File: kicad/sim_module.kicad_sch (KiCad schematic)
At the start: 2 parts, among them J40 693043020611, U40 TPD3F303DPVR

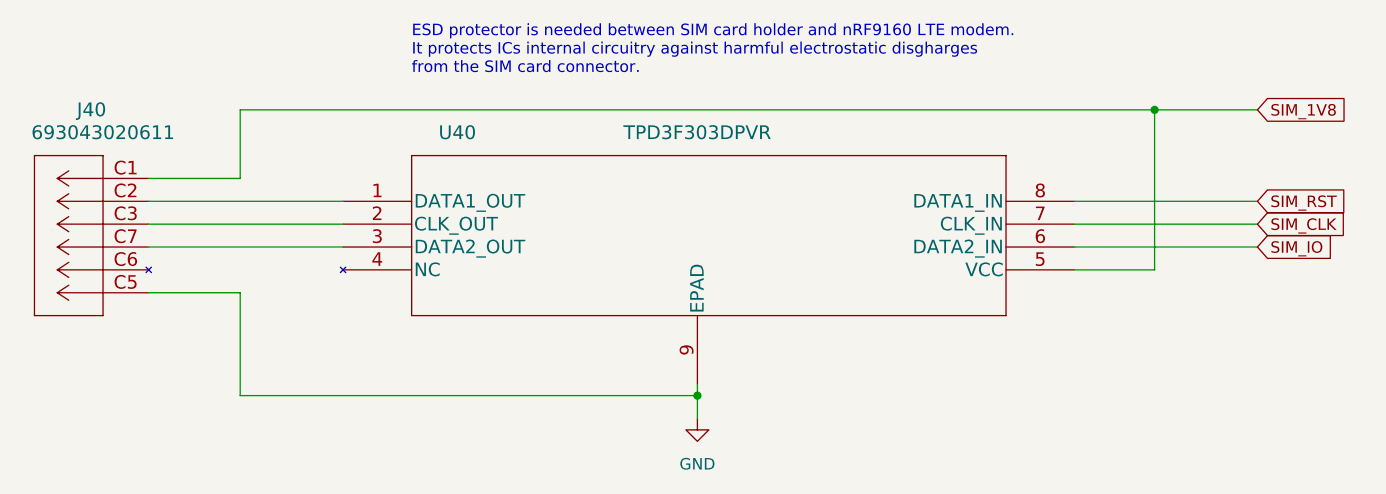
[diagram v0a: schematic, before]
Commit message: ESD change
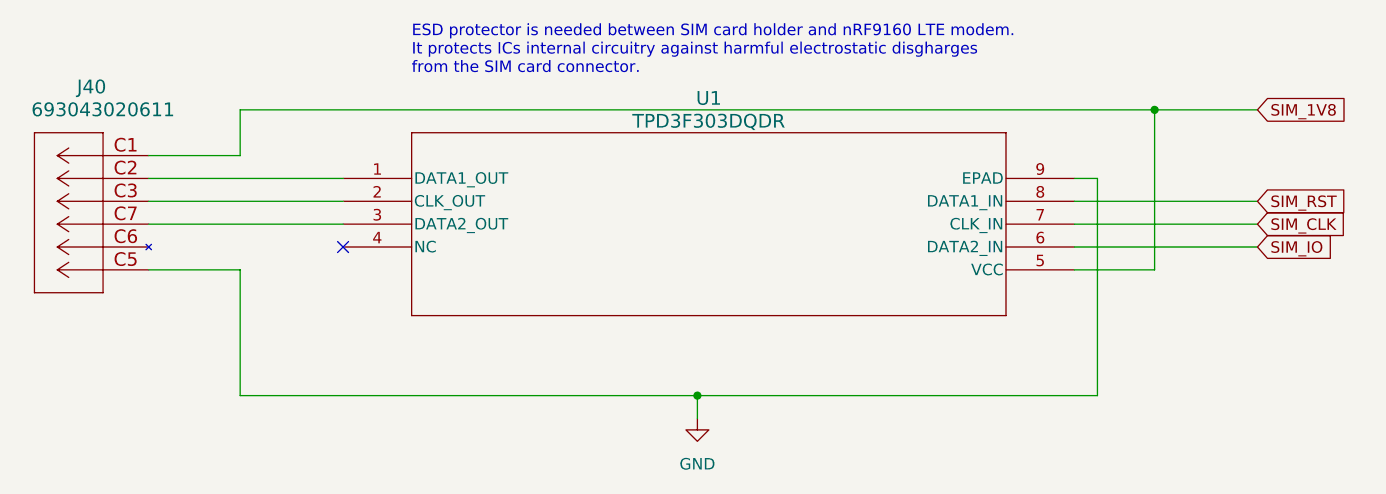
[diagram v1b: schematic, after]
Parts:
- removed U40: TPD3F303DPVR, TPD3F303DPVR:TPD3F303DPVR, symbol TPD3F303DPVR:TPD3F303DPVR
- added U1: TPD3F303DQDR, TPD3F303DQDR:TPD3F303DQDR, symbol TPD3F303DQDR:TPD3F303DQDR
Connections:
- net GND: now also U1.9 (EPAD)
- net SIM_1V8: now also U1.5 (VCC)
- net SIM_CLK: now also U1.7 (CLK_IN)
- net SIM_IO: now also U1.6 (DATA2_IN)
- net SIM_RST: now also U1.8 (DATA1_IN)
- net at J40.C2: now also U1.1 (DATA1_OUT)
- net at J40.C3: now also U1.2 (CLK_OUT)
- net at J40.C7: now also U1.3 (DATA2_OUT)
- no-connect marks 0 -> 1
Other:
- moved on the sheet: J40
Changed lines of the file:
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@@
   (junction (at 106.68 73.66) (diameter 0) (color 0 0 0 0)
   )
-  (wire (pts (xy 55.88 62.23) (xy 55.88 73.66))
+  (no_connect (at 67.31 57.15))
+  (wire (pts (xy 45.72 49.53) (xy 67.31 49.53))
+    (stroke (width 0) (type default))
+  )
+  (wire (pts (xy 55.88 59.69) (xy 55.88 73.66))
     (stroke (width 0) (type default))
   )
@@
     (stroke (width 0) (type default))
   )
-  (wire (pts (xy 45.72 49.53) (xy 55.88 49.53))
+  (wire (pts (xy 45.72 46.99) (xy 55.88 46.99))
+    (stroke (width 0) (type default))
+  )
+  (wire (pts (xy 148.59 49.53) (xy 151.13 49.53))
     (stroke (width 0) (type default))
   )
@@
     (stroke (width 0) (type default))
   )
+  (wire (pts (xy 45.72 52.07) (xy 67.31 52.07))
+    (stroke (width 0) (type default))
+  )
   (wire (pts (xy 55.88 41.91) (xy 157.48 41.91))
     (stroke (width 0) (type default))
   )
-  (wire (pts (xy 45.72 52.07) (xy 67.31 52.07))
+  (wire (pts (xy 151.13 73.66) (xy 106.68 73.66))
     (stroke (width 0) (type default))
   )
@@
     (stroke (width 0) (type default))
   )
-  (wire (pts (xy 55.88 49.53) (xy 55.88 41.91))
+  (wire (pts (xy 55.88 59.69) (xy 45.72 59.69))
     (stroke (width 0) (type default))
   )
-  (wire (pts (xy 45.72 57.15) (xy 67.31 57.15))
+  (wire (pts (xy 55.88 41.91) (xy 55.88 46.99))
     (stroke (width 0) (type default))
   )
-  (wire (pts (xy 106.68 72.39) (xy 106.68 73.66))
+  (wire (pts (xy 151.13 49.53) (xy 151.13 73.66))
     (stroke (width 0) (type default))
   )
   (wire (pts (xy 106.68 73.66) (xy 106.68 76.2))
-    (stroke (width 0) (type default))
-  )
-  (wire (pts (xy 45.72 62.23) (xy 55.88 62.23))
     (stroke (width 0) (type default))
   )
@@
     )
   )
-  (symbol (lib_id "693043020611:693043020611") (at 45.72 49.53 0) (mirror y) (unit 1)
+  (symbol (lib_id "693043020611:693043020611") (at 45.72 46.99 0) (mirror y) (unit 1)
     (in_bom yes) (on_board yes) (dnp no)
-    (property "Reference" "J40" (at 39.37 41.91 0)
+    (property "Reference" "J40" (at 39.37 39.37 0)
       (effects (font (size 1.524 1.524)))
     )
-    (property "Value" "693043020611" (at 40.64 44.45 0)
+    (property "Value" "693043020611" (at 40.64 41.91 0)
       (effects (font (size 1.524 1.524)))
     )
-    (property "Footprint" "693043020611:693043020611" (at 35.56 42.926 0)
+    (property "Footprint" "693043020611:693043020611" (at 35.56 40.386 0)
       (effects (font (size 1.524 1.524)) hide)
     )
-    (property "Datasheet" "" (at 45.72 49.53 0)
+    (property "Datasheet" "" (at 45.72 46.99 0)
       (effects (font (size 1.524 1.524)))
     )
-    (property "Digikey" "296-28299-1-ND" (at 45.72 49.53 0)
+    (property "Digikey" "296-28299-1-ND" (at 45.72 46.99 0)
       (effects (font (size 1.27 1.27)) hide)
     )
@@
         (path "/184b47ed-2c2b-4c02-be35-d18f4f4e5685/38627e9e-7096-4a1a-bc9e-0f2735fcbe8c"
           (reference "J40") (unit 1)
-        )
-      )
-    )
-  )
-  (symbol (lib_id "TPD3F303DPVR:TPD3F303DPVR") (at 67.31 52.07 0) (unit 1)
-    (in_bom yes) (on_board yes) (dnp no)
-    (property "Reference" "U40" (at 80.01 44.45 0)
-      (effects (font (size 1.524 1.524)))
-    )
-    (property "Value" "TPD3F303DPVR" (at 106.68 44.45 0)
-      (effects (font (size 1.524 1.524)))
-    )
-    (property "Footprint" "TPD3F303DPVR:TPD3F303DPVR" (at 26.67 58.166 0)
-      (effects (font (size 1.524 1.524)) hide)
-    )
-    (property "Datasheet" "" (at 67.31 52.07 0)
-      (effects (font (size 1.524 1.524)))
-    )
-    (property "Digikey" "732-5954-1-ND" (at 67.31 52.07 0)
-      (effects (font (size 1.27 1.27)) hide)
-    )
-    (pin "1")
-    (pin "2")
-    (pin "3")
-    (pin "4")
-    (pin "5")
-    (pin "6")
-    (pin "7")
-    (pin "8")
-    (pin "9")
-    (instances
-      (project "IoT_sulari"
-        (path "/184b47ed-2c2b-4c02-be35-d18f4f4e5685/38627e9e-7096-4a1a-bc9e-0f2735fcbe8c"
-          (reference "U40") (unit 1)
         )
       )
@@
         )
       )
+    )
+  )
+  (symbol (lib_id "TPD3F303DQDR:TPD3F303DQDR") (at 67.31 49.53 0) (unit 1)
+    (in_bom yes) (on_board yes) (dnp no) (fields_autoplaced)
+    (property "Reference" "U1" (at 107.95 40.64 0)
+      (effects (font (size 1.524 1.524)))
+    )
+    (property "Value" "TPD3F303DQDR" (at 107.95 43.18 0)
+      (effects (font (size 1.524 1.524)))
+    )
+    (property "Footprint" "TPD3F303DQDR:TPD3F303DQDR" (at 67.31 49.53 0)
+      (effects (font (size 1.27 1.27) italic) hide)
+    )
+    (property "Datasheet" "TPD3F303DQDR" (at 67.31 49.53 0)
+      (effects (font (size 1.27 1.27) italic) hide)
+    )
+    (pin "1")
+    (pin "2")
+    (pin "3")
+    (pin "4")
+    (pin "5")
+    (pin "6")
+    (pin "7")
+    (pin "8")
+    (pin "9")
+    (instances
+      (project "IoT_sulari"
+        (path "/184b47ed-2c2b-4c02-be35-d18f4f4e5685/38627e9e-7096-4a1a-bc9e-0f2735fcbe8c"
+          (reference "U1") (unit 1)
+        )
+      )

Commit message: Revert "ESD change"
This reverts commit acabe66db7bce87ed7ccd6d28b87d0a8866a87e9.
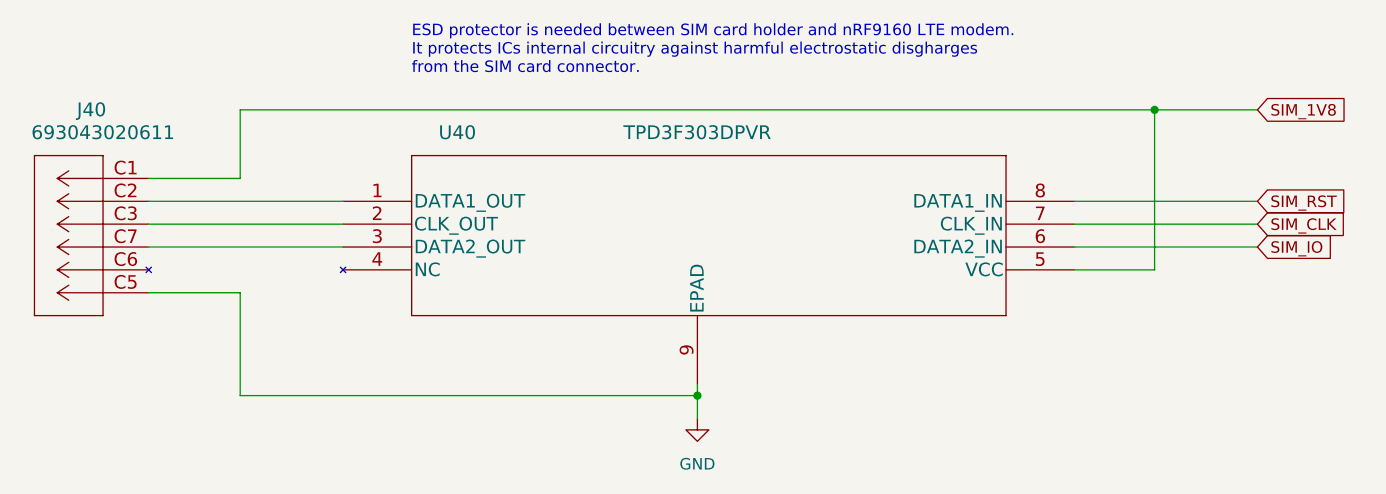
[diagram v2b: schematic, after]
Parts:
- removed U1: TPD3F303DQDR, TPD3F303DQDR:TPD3F303DQDR, symbol TPD3F303DQDR:TPD3F303DQDR
- added U40: TPD3F303DPVR, TPD3F303DPVR:TPD3F303DPVR, symbol TPD3F303DPVR:TPD3F303DPVR
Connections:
- net GND: now also U40.9 (EPAD)
- net SIM_1V8: now also U40.5 (VCC)
- net SIM_CLK: now also U40.7 (CLK_IN)
- net SIM_IO: now also U40.6 (DATA2_IN)
- net SIM_RST: now also U40.8 (DATA1_IN)
- net at J40.C2: now also U40.1 (DATA1_OUT)
- net at J40.C3: now also U40.2 (CLK_OUT)
- net at J40.C7: now also U40.3 (DATA2_OUT)
- no-connect marks 1 -> 0
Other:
- moved on the sheet: J40
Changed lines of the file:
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@@
   (junction (at 106.68 73.66) (diameter 0) (color 0 0 0 0)
   )
-  (no_connect (at 67.31 57.15))
-  (wire (pts (xy 45.72 49.53) (xy 67.31 49.53))
-    (stroke (width 0) (type default))
-  )
-  (wire (pts (xy 55.88 59.69) (xy 55.88 73.66))
+  (wire (pts (xy 55.88 62.23) (xy 55.88 73.66))
     (stroke (width 0) (type default))
   )
@@
     (stroke (width 0) (type default))
   )
-  (wire (pts (xy 45.72 46.99) (xy 55.88 46.99))
-    (stroke (width 0) (type default))
-  )
-  (wire (pts (xy 148.59 49.53) (xy 151.13 49.53))
+  (wire (pts (xy 45.72 49.53) (xy 55.88 49.53))
     (stroke (width 0) (type default))
   )
@@
     (stroke (width 0) (type default))
   )
-  (wire (pts (xy 45.72 52.07) (xy 67.31 52.07))
-    (stroke (width 0) (type default))
-  )
   (wire (pts (xy 55.88 41.91) (xy 157.48 41.91))
     (stroke (width 0) (type default))
   )
-  (wire (pts (xy 151.13 73.66) (xy 106.68 73.66))
+  (wire (pts (xy 45.72 52.07) (xy 67.31 52.07))
     (stroke (width 0) (type default))
   )
@@
     (stroke (width 0) (type default))
   )
-  (wire (pts (xy 55.88 59.69) (xy 45.72 59.69))
+  (wire (pts (xy 55.88 49.53) (xy 55.88 41.91))
     (stroke (width 0) (type default))
   )
-  (wire (pts (xy 55.88 41.91) (xy 55.88 46.99))
+  (wire (pts (xy 45.72 57.15) (xy 67.31 57.15))
     (stroke (width 0) (type default))
   )
-  (wire (pts (xy 151.13 49.53) (xy 151.13 73.66))
+  (wire (pts (xy 106.68 72.39) (xy 106.68 73.66))
     (stroke (width 0) (type default))
   )
   (wire (pts (xy 106.68 73.66) (xy 106.68 76.2))
+    (stroke (width 0) (type default))
+  )
+  (wire (pts (xy 45.72 62.23) (xy 55.88 62.23))
     (stroke (width 0) (type default))
   )
@@
     )
   )
-  (symbol (lib_id "693043020611:693043020611") (at 45.72 46.99 0) (mirror y) (unit 1)
+  (symbol (lib_id "693043020611:693043020611") (at 45.72 49.53 0) (mirror y) (unit 1)
     (in_bom yes) (on_board yes) (dnp no)
-    (property "Reference" "J40" (at 39.37 39.37 0)
+    (property "Reference" "J40" (at 39.37 41.91 0)
       (effects (font (size 1.524 1.524)))
     )
-    (property "Value" "693043020611" (at 40.64 41.91 0)
+    (property "Value" "693043020611" (at 40.64 44.45 0)
       (effects (font (size 1.524 1.524)))
     )
-    (property "Footprint" "693043020611:693043020611" (at 35.56 40.386 0)
+    (property "Footprint" "693043020611:693043020611" (at 35.56 42.926 0)
       (effects (font (size 1.524 1.524)) hide)
     )
-    (property "Datasheet" "" (at 45.72 46.99 0)
+    (property "Datasheet" "" (at 45.72 49.53 0)
       (effects (font (size 1.524 1.524)))
     )
-    (property "Digikey" "296-28299-1-ND" (at 45.72 46.99 0)
+    (property "Digikey" "296-28299-1-ND" (at 45.72 49.53 0)
       (effects (font (size 1.27 1.27)) hide)
     )
@@
         (path "/184b47ed-2c2b-4c02-be35-d18f4f4e5685/38627e9e-7096-4a1a-bc9e-0f2735fcbe8c"
           (reference "J40") (unit 1)
+        )
+      )
+    )
+  )
+  (symbol (lib_id "TPD3F303DPVR:TPD3F303DPVR") (at 67.31 52.07 0) (unit 1)
+    (in_bom yes) (on_board yes) (dnp no)
+    (property "Reference" "U40" (at 80.01 44.45 0)
+      (effects (font (size 1.524 1.524)))
+    )
+    (property "Value" "TPD3F303DPVR" (at 106.68 44.45 0)
+      (effects (font (size 1.524 1.524)))
+    )
+    (property "Footprint" "TPD3F303DPVR:TPD3F303DPVR" (at 26.67 58.166 0)
+      (effects (font (size 1.524 1.524)) hide)
+    )
+    (property "Datasheet" "" (at 67.31 52.07 0)
+      (effects (font (size 1.524 1.524)))
+    )
+    (property "Digikey" "732-5954-1-ND" (at 67.31 52.07 0)
+      (effects (font (size 1.27 1.27)) hide)
+    )
+    (pin "1")
+    (pin "2")
+    (pin "3")
+    (pin "4")
+    (pin "5")
+    (pin "6")
+    (pin "7")
+    (pin "8")
+    (pin "9")
+    (instances
+      (project "IoT_sulari"
+        (path "/184b47ed-2c2b-4c02-be35-d18f4f4e5685/38627e9e-7096-4a1a-bc9e-0f2735fcbe8c"
+          (reference "U40") (unit 1)
         )
       )
@@
         )
       )
-    )
-  )
-  (symbol (lib_id "TPD3F303DQDR:TPD3F303DQDR") (at 67.31 49.53 0) (unit 1)
-    (in_bom yes) (on_board yes) (dnp no) (fields_autoplaced)
-    (property "Reference" "U1" (at 107.95 40.64 0)
-      (effects (font (size 1.524 1.524)))
-    )
-    (property "Value" "TPD3F303DQDR" (at 107.95 43.18 0)
-      (effects (font (size 1.524 1.524)))
-    )
-    (property "Footprint" "TPD3F303DQDR:TPD3F303DQDR" (at 67.31 49.53 0)
-      (effects (font (size 1.27 1.27) italic) hide)
-    )
-    (property "Datasheet" "TPD3F303DQDR" (at 67.31 49.53 0)
-      (effects (font (size 1.27 1.27) italic) hide)
-    )
-    (pin "1")
-    (pin "2")
-    (pin "3")
-    (pin "4")
-    (pin "5")
-    (pin "6")
-    (pin "7")
-    (pin "8")
-    (pin "9")
-    (instances
-      (project "IoT_sulari"
-        (path "/184b47ed-2c2b-4c02-be35-d18f4f4e5685/38627e9e-7096-4a1a-bc9e-0f2735fcbe8c"
-          (reference "U1") (unit 1)
-        )
-      )
